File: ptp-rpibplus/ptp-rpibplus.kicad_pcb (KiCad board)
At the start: 2 copper layers, 6 parts, among them J1 RASPI_B+, J2 MODULE_HEADER, J3 MODULE_HEADER

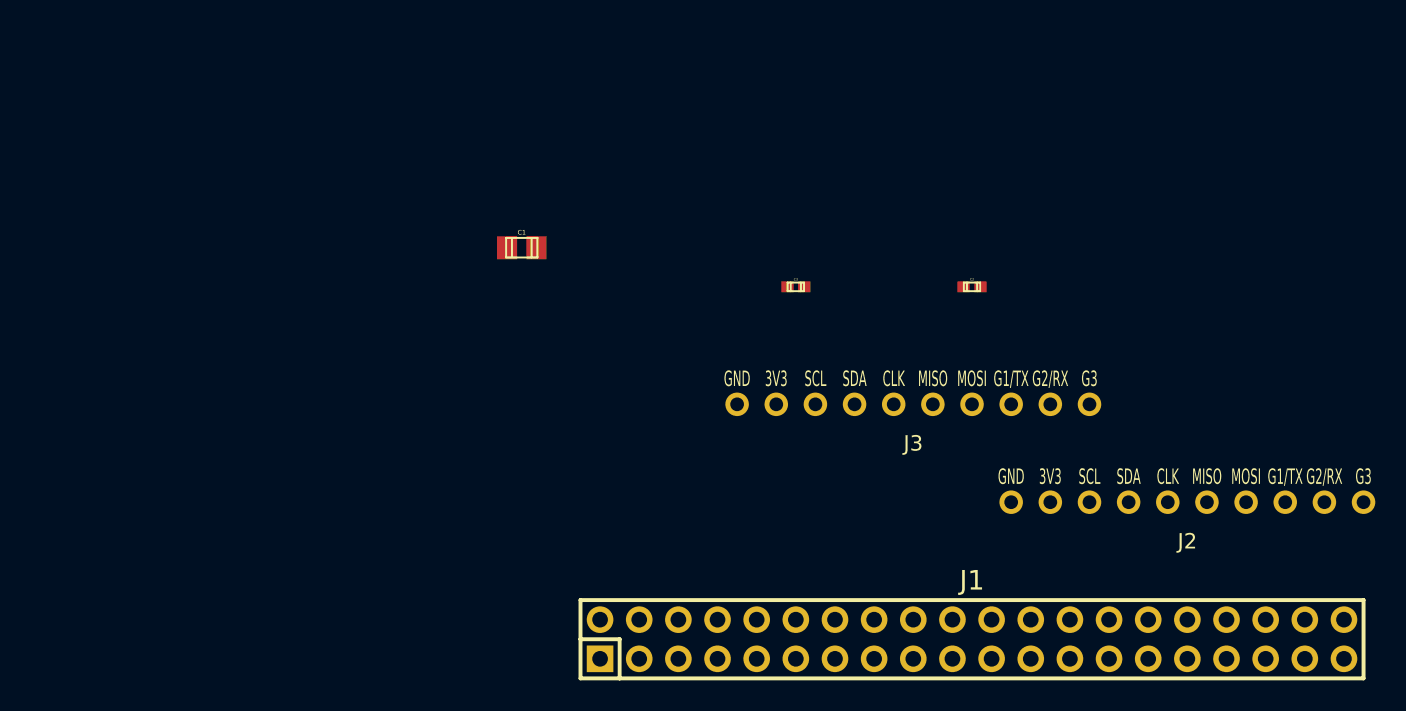
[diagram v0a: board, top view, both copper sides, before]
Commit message: ...at least the board has mount holes now
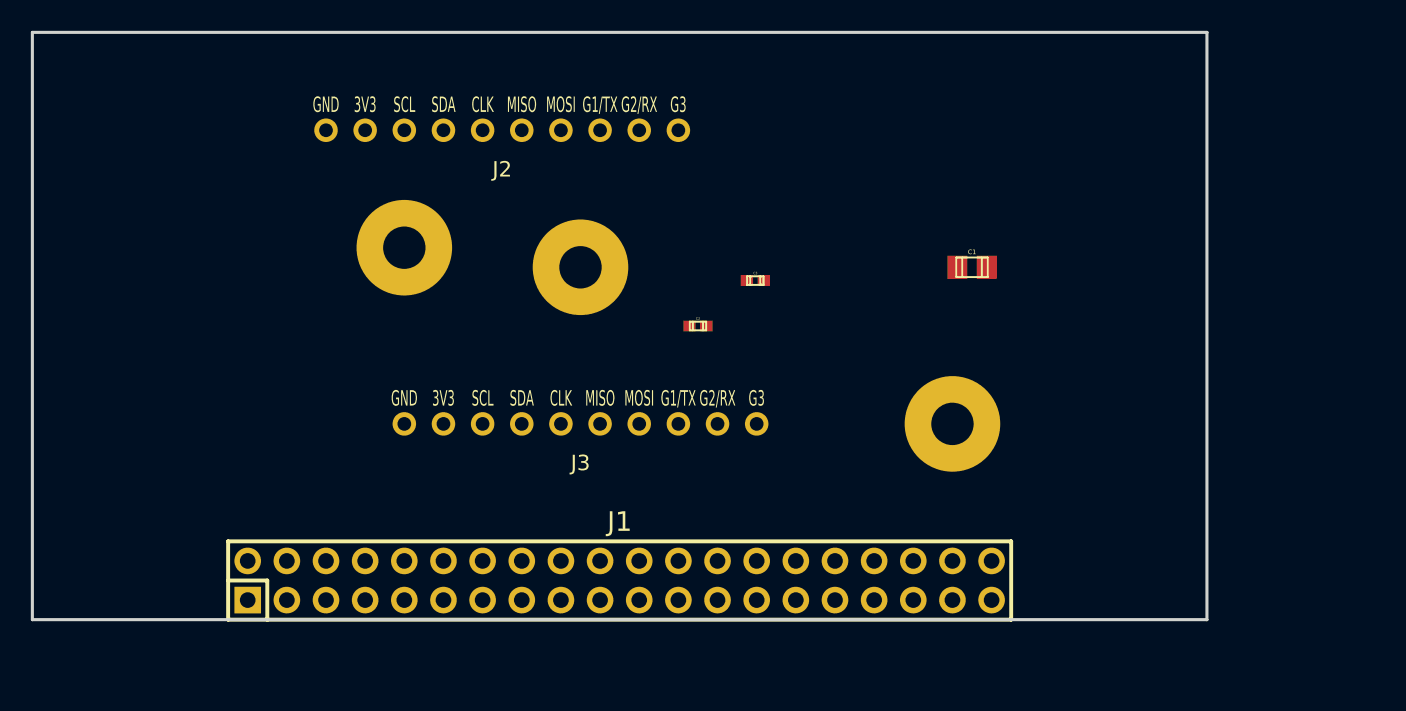
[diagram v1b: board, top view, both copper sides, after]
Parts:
- added H1: HOLE, parts:HOLE-2.75mm-6.2mm, F.Cu at (125.7, 102.9)
- added H2: HOLE, parts:HOLE-2.75mm-6.2mm, F.Cu at (137.2, 104.1)
- added H3: HOLE, parts:HOLE-2.75mm-6.2mm, F.Cu at (161.3, 114.3)
- moved J2 50.6 mm to (132.1, 95.2)
- moved C1 29.2 mm to (162.6, 104.1)
- moved J1 23.2 mm to (139.7, 124.5)
- moved J3 21.6 mm to (137.2, 114.3)
- moved C2 18.0 mm to (144.8, 108.0)
- moved C3 2.66 mm to (148.5, 105.0)
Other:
- board outline added: 76.2 x 38.1 mm
- net class Default: clearance 0.2032 -> 0.254; trace_width 0.2032 -> 0.254
- rule trace_clearance: 0.2032 -> 0.254
- rule trace_min: 0.2032 -> 0.254
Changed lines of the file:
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@@
   (general
     (links 33)
-    (no_connects 33)
-    (area 131.49326 101.324156 188.976 131.191001)
+    (no_connects 22)
+    (area 0 0 0 0)
     (thickness 1.6)
-    (drawings 0)
+    (drawings 4)
     (tracks 0)
     (zones 0)
-    (modules 6)
+    (modules 9)
     (nets 34)
   )
@@
   )
   (setup
-    (last_trace_width 0.2032)
-    (trace_clearance 0.2032)
+    (last_trace_width 0.254)
+    (trace_clearance 0.254)
     (zone_clearance 0.508)
     (zone_45_only no)
-    (trace_min 0.2032)
+    (trace_min 0.254)
     (segment_width 0.2)
     (edge_width 0.1)
@@
   (net 33 /CLK)
   (net_class Default "This is the default net class."
-    (clearance 0.2032)
-    (trace_width 0.2032)
+    (clearance 0.254)
+    (trace_width 0.254)
     (via_dia 0.889)
     (via_drill 0.635)
@@
   )
   (module Capacitors_SMD:c_0805 (layer F.Cu)
-    (at 133.35 102.87)
+    (at 162.56 104.14)
     (descr "SMT capacitor, 0805")
     (fp_text reference C1 (at 0 -0.9906) (layer F.SilkS)
@@
   )
   (module Capacitors_SMD:c_0402 (layer F.Cu)
-    (at 162.56 105.41)
+    (at 144.78 107.95)
     (descr "SMT capacitor, 0402")
     (fp_text reference C2 (at 0 -0.4826) (layer F.SilkS)
@@
   )
   (module Capacitors_SMD:c_0402 (layer F.Cu)
-    (at 151.13 105.41)
+    (at 148.5011 105.0036)
     (descr "SMT capacitor, 0402")
     (fp_text reference C3 (at 0 -0.4826) (layer F.SilkS)
@@
     )
   )
+  (module parts:HOLE-2.75mm-6.2mm (layer F.Cu)
+    (at 125.73 102.87)
+    (fp_text reference H1 (at 0 -5.08) (layer F.SilkS) hide
+      (effects (font (size 1 1) (thickness 0.15)))
+    )
+    (fp_text value HOLE (at 0 5.08) (layer F.SilkS) hide
+      (effects (font (size 1 1) (thickness 0.15)))
+    )
+    (pad "" np_thru_hole circle (at 0 0) (size 6.2 6.2) (drill 2.75) (layers *.Cu *.Mask F.SilkS))
+  )
+  (module parts:HOLE-2.75mm-6.2mm (layer F.Cu)
+    (at 137.16 104.14)
+    (fp_text reference H2 (at 0 -5.08) (layer F.SilkS) hide
+      (effects (font (size 1 1) (thickness 0.15)))
+    )
+    (fp_text value HOLE (at 0 5.08) (layer F.SilkS) hide
+      (effects (font (size 1 1) (thickness 0.15)))
+    )
+    (pad "" np_thru_hole circle (at 0 0) (size 6.2 6.2) (drill 2.75) (layers *.Cu *.Mask F.SilkS))
+  )
+  (module parts:HOLE-2.75mm-6.2mm (layer F.Cu)
+    (at 161.29 114.3)
+    (fp_text reference H3 (at 0 -5.08) (layer F.SilkS) hide
+      (effects (font (size 1 1) (thickness 0.15)))
+    )
+    (fp_text value HOLE (at 0 5.08) (layer F.SilkS) hide
+      (effects (font (size 1 1) (thickness 0.15)))
+    )
+    (pad "" np_thru_hole circle (at 0 0) (size 6.2 6.2) (drill 2.75) (layers *.Cu *.Mask F.SilkS))
+  )
   (module Pin_Headers:Pin_Header_Straight_2x20 (layer F.Cu)
-    (at 162.56 128.27)
+    (at 139.7 124.46)
     (descr "1 pin")
     (tags "CONN DEV")
@@
   )
   (module parts:MODULE_HEADER_TESSEL (layer F.Cu)
-    (at 176.53 119.38)
+    (at 132.08 95.25)
     (fp_text reference J2 (at 0 2.54) (layer F.SilkS)
       (effects (font (size 1 1) (thickness 0.1)))
@@
   )
   (module parts:MODULE_HEADER_TESSEL (layer F.Cu)
-    (at 158.75 113.03)
+    (at 137.16 114.3)
     (fp_text reference J3 (at 0 2.54) (layer F.SilkS)
       (effects (font (size 1 1) (thickness 0.1)))
@@
       (net 13 /B_G3))
   )
+  (gr_line (start 101.6 88.9) (end 101.6 127) (layer Edge.Cuts) (width 0.2))
+  (gr_line (start 177.8 88.9) (end 101.6 88.9) (layer Edge.Cuts) (width 0.2))
+  (gr_line (start 177.8 127) (end 177.8 88.9) (layer Edge.Cuts) (width 0.2))
+  (gr_line (start 101.6 127) (end 177.8 127) (layer Edge.Cuts) (width 0.2))
 )
